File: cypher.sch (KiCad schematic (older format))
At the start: 30 parts, among them J2 AVR-ISP-6, J3 Breakout, Q1 MMBT3904, SW1 SW_Push, U1 ATmega32U4-MU, U2 PRTR5V0U2X, Y1 16Mhz

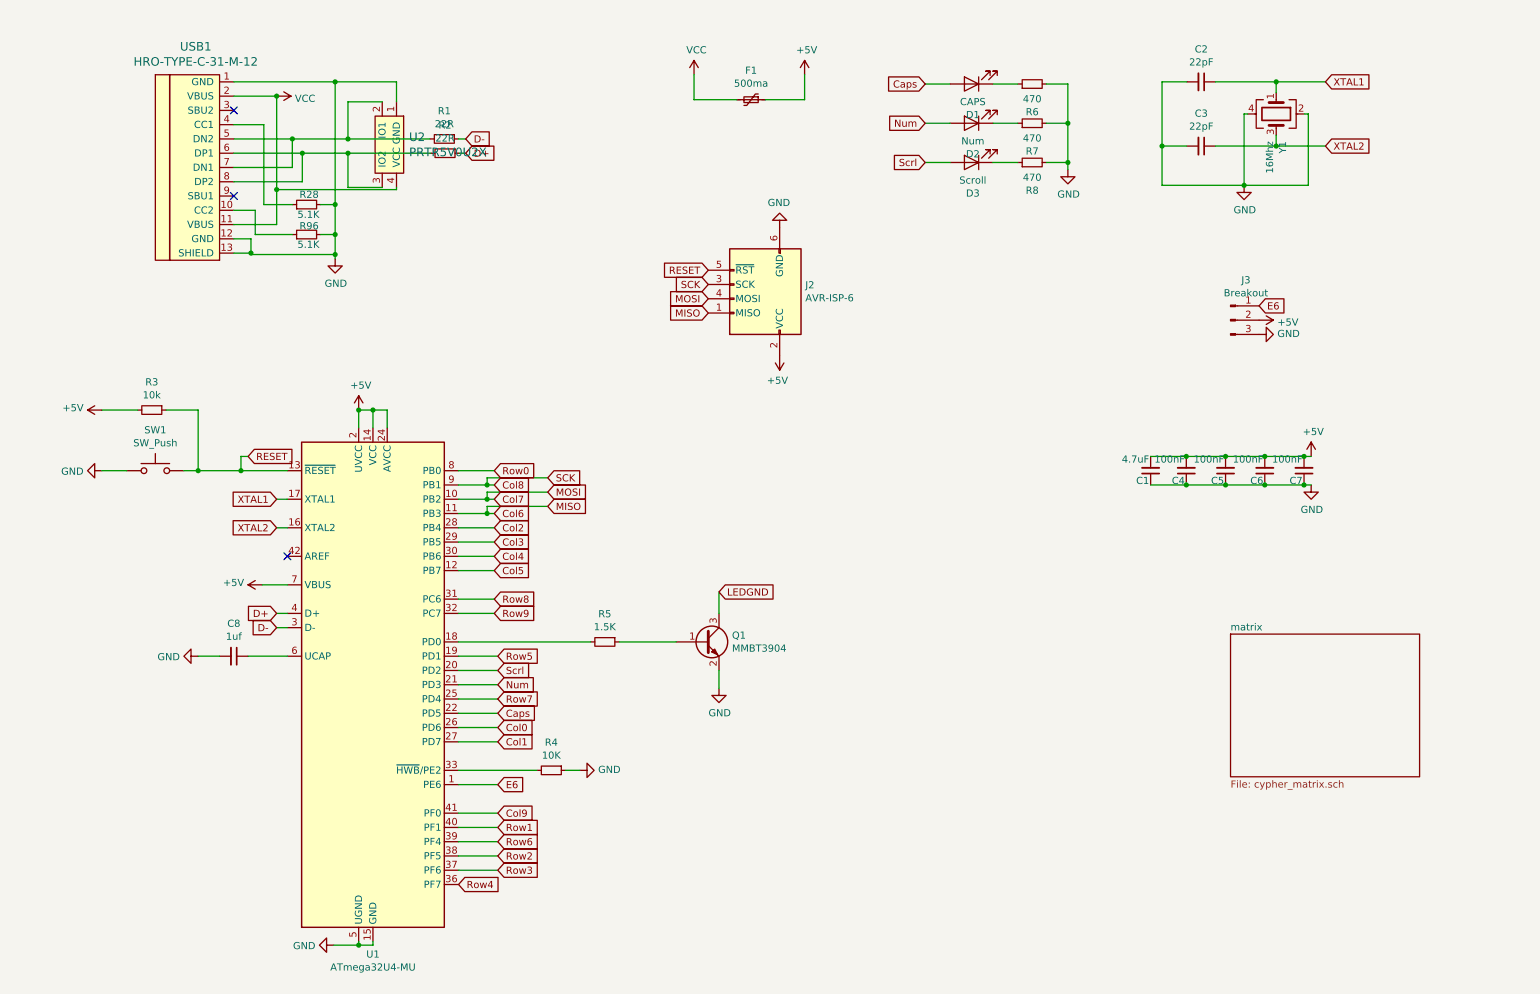
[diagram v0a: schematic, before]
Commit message: Added base for Rev 6
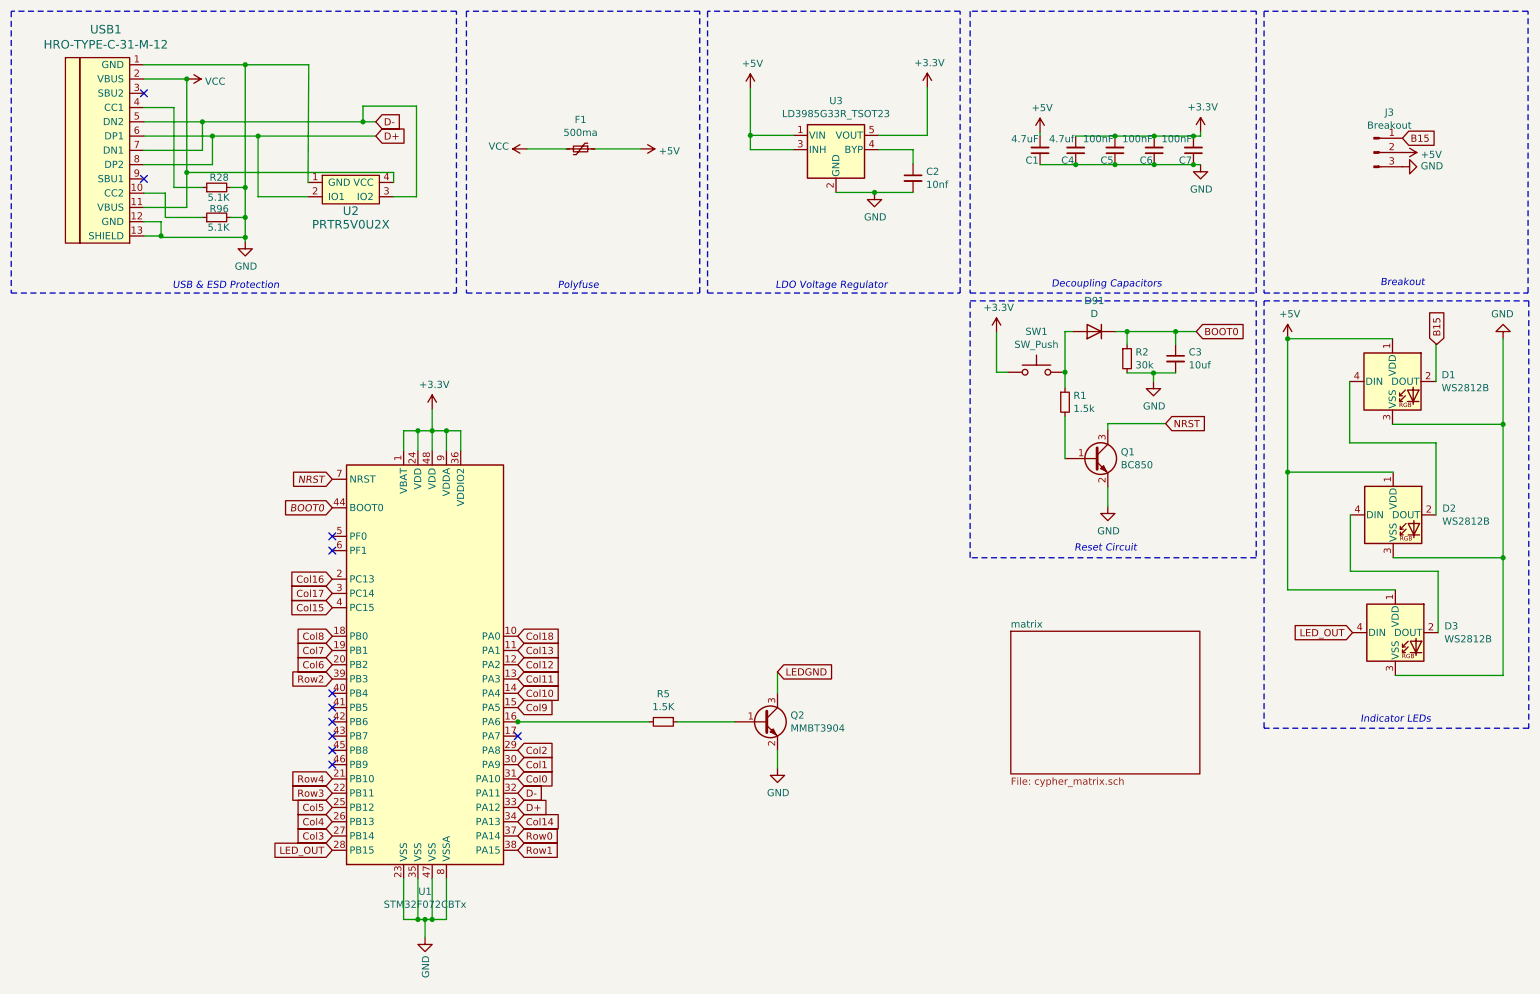
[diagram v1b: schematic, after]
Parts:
- removed C8: 1uf, Capacitor_SMD:C_0603_1608Metric, symbol Device:C_Small
- removed D1: CAPS, LED_THT:LED_D1.8mm_W3.3mm_H2.4mm, symbol Device:LED
- removed D2: Num, LED_THT:LED_D1.8mm_W3.3mm_H2.4mm, symbol Device:LED
- removed D3: Scroll, LED_THT:LED_D1.8mm_W3.3mm_H2.4mm, symbol Device:LED
- removed J2: AVR-ISP-6, Connector_PinHeader_2.54mm:PinHeader_2x03_P2.54mm_Vertical, symbol Connector:AVR-ISP-6
- removed Q1: MMBT3904, Package_TO_SOT_SMD:SOT-23, symbol transistors:MMBT3904
- removed R3: 10k, Resistor_SMD:R_0603_1608Metric, symbol Device:R_Small
- removed R4: 10K, Resistor_SMD:R_0603_1608Metric, symbol Device:R_Small
- removed R6, R7, R8: 470, Resistor_SMD:R_0603_1608Metric, symbol Device:R_Small
- removed U1: ATmega32U4-MU, Package_DFN_QFN:QFN-44-1EP_7x7mm_P0.5mm_EP5.2x5.2mm, symbol MCU_Microchip_ATmega:ATmega32U4-MU
- removed U2: PRTR5V0U2X, PRTR5V0U2X:SOT143B, symbol ai03-locallib:PRTR5V0U2X
- removed Y1: 16Mhz, Crystal:Crystal_SMD_2520-4Pin_2.5x2.0mm, symbol Device:Crystal_GND24
- added D1, D2, D3: WS2812B, CrumpPrints:WS2812-2020, symbol LED:WS2812B
- added D91: D, Diode_SMD:D_0603_1608Metric, symbol Device:D
- added Q1: BC850, Package_TO_SOT_SMD:SOT-23, symbol Transistor_BJT:BC850
- added Q2: MMBT3904, Package_TO_SOT_SMD:SOT-23, symbol Transistor_BJT:MMBT3904
- added U1: STM32F072CBTx, Package_QFP:LQFP-48_7x7mm_P0.5mm, symbol MCU_ST_STM32F0:STM32F072CBTx
- added U2: PRTR5V0U2X, random-keyboard-parts:SOT143B, symbol random-keyboard-parts:PRTR5V0U2X
- added U3: LD3985G33R_TSOT23, Package_TO_SOT_SMD:TSOT-23-5, symbol Regulator_Linear:LD3985G33R_TSOT23
- C2: value 22pF -> 10nf
- C3: value 22pF -> 10uf
- C4: value 100nF -> 4.7uf
- F1: footprint Fuse:Fuse_0805_2012Metric -> Fuse:Fuse_0603_1608Metric
- R1: value 22R -> 1.5k
- R2: value 22R -> 30k
- SW1: footprint Connector_PinHeader_2.54mm:PinHeader_2x01_P2.54mm_Vertical -> reset:ResetShort
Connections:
- net +5V: now also D1.1 (VDD), D2.1 (VDD), D3.1 (VDD), U3.1 (VIN), U3.3 (INH); no longer C4.2, C5.2, C6.2, C7.2
- net Col0: now also U1.31 (PA10)
- net Col1: now also U1.30 (PA9)
- net Col2: now also U1.29 (PA8)
- net Col3: now also U1.27 (PB14)
- net Col4: now also U1.26 (PB13)
- net Col5: now also U1.25 (PB12)
- net Col6: now also U1.20 (PB2)
- net Col7: now also U1.19 (PB1)
- net Col8: now also U1.18 (PB0)
- net Col9: now also U1.15 (PA5)
- net D+: now also USB1.6 (DP1), USB1.8 (DP2), U1.33 (PA12), U2.2 (IO1); no longer R2.1
- net D-: now also USB1.5 (DN2), USB1.7 (DN1), U1.32 (PA11), U2.3 (IO2); no longer R1.1
- net GND: now also R2.2, D1.3 (VSS), D2.3 (VSS), D3.3 (VSS), Q1.2 (E), Q2.2 (E), U1.23 (VSS), U1.35 (VSS), U1.47 (VSS), U1.8 (VSSA), U2.1 (GND), U3.2 (GND); no longer SW1.1
- net LEDGND: now also Q2.3 (C)
- net Row0: now also U1.37 (PA14)
- net Row1: now also U1.38 (PA15)
- net Row2: now also U1.39 (PB3)
- net Row3: now also U1.22 (PB11)
- net Row4: now also U1.21 (PB10)
- net VCC: now also U2.4 (VCC)
- net at R5.1: now also Q2.1 (B)
- net at R5.2: now also U1.16 (PA6)
- net E6 renamed B15
- net B15: now also D1.2 (DOUT)
- net RESET: no longer names the net of SW1.2
- net RESET: now also R1.1, D91.2 (A)
- net XTAL1: no longer names the net of C2.1
- net XTAL1: now also U3.4 (BYP)
- net XTAL2 renamed BOOT0
- net BOOT0: now also R2.1, D91.1 (K), U1.44 (BOOT0)
- new net: Q1.1 (B), R1.2
- new net: D1.4 (DIN), D2.2 (DOUT)
- new net: D2.4 (DIN), D3.2 (DOUT)
- new net +3V3: C4.2, C5.2, C6.2, C7.2, SW1.1, U1.1 (VBAT), U1.24 (VDD), U1.36 (VDDIO2), U1.48 (VDD), U1.9 (VDDA), U3.5 (VOUT)
- new net Col10: U1.14 (PA4)
- new net Col11: U1.13 (PA3)
- new net Col12: U1.12 (PA2)
- new net Col13: U1.11 (PA1)
- new net Col14: U1.34 (PA13)
- new net Col15: U1.4 (PC15)
- new net Col16: U1.2 (PC13)
- new net Col17: U1.3 (PC14)
- new net Col18: U1.10 (PA0)
- new net LED_OUT: D3.4 (DIN), U1.28 (PB15)
- new net NRST: Q1.3 (C), U1.7 (NRST)
- no-connect marks 3 -> 11
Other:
- note added: "Breakout\n"
- note added: "Decoupling Capacitors\n"
- note added: "Indicator LEDs\n"
- note added: "LDO Voltage Regulator\n\n"
- note added: "Polyfuse\n"
- note added: "Reset Circuit\n"
- note added: "USB & ESD Protection\n"
- moved on the sheet: C1, C4, C5, C6, C7, J3, R28, R5, R96, USB1

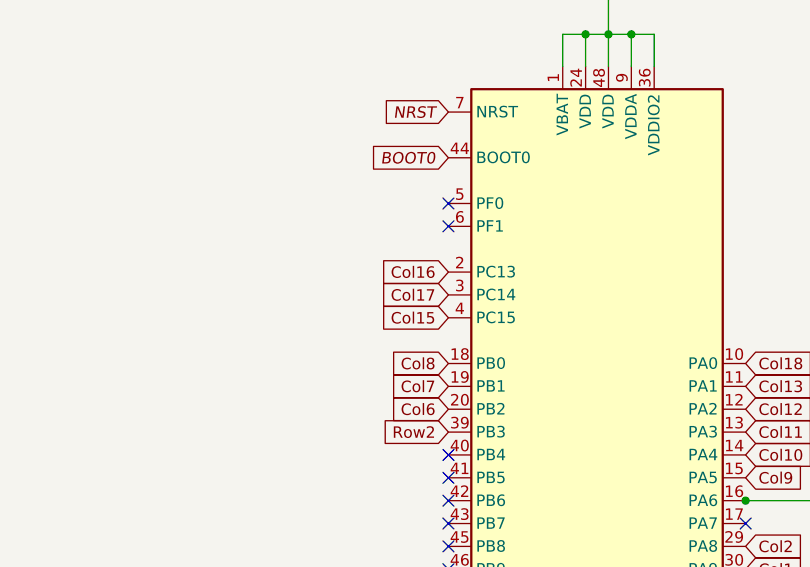
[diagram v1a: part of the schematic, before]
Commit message: Rerouted, added render
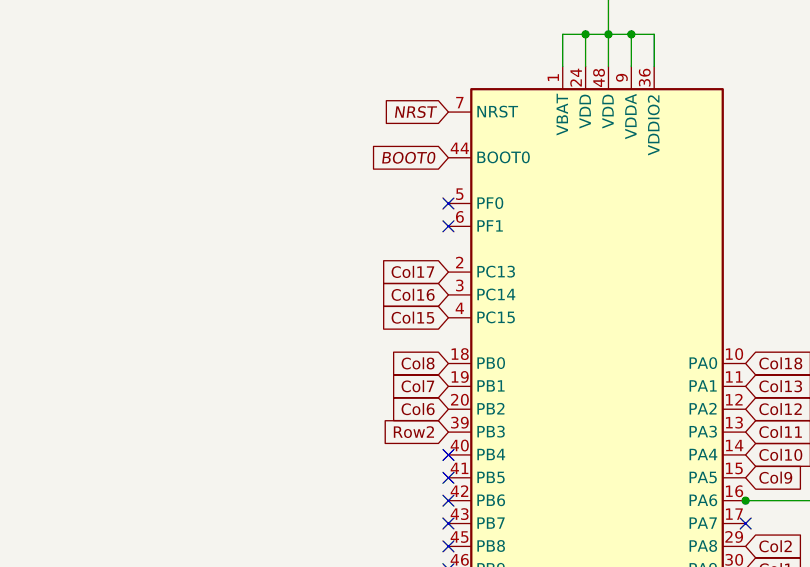
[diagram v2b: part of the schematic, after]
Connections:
- net Col16: now also U1.3 (PC14); no longer U1.2 (PC13)
- net Col17: now also U1.2 (PC13); no longer U1.3 (PC14)
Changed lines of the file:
@@
 Text GLabel 2780 4755 0    50   Input ~ 0
 Col15
+Text GLabel 2780 4655 0    50   Input ~ 0
+Col16
 Text GLabel 2780 4555 0    50   Input ~ 0
-Col16
-Text GLabel 2780 4655 0    50   Input ~ 0
 Col17
 Text GLabel 4080 4955 2    50   Input ~ 0
